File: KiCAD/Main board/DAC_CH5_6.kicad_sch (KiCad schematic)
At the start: 51 parts, among them U1 PCM1789-Q1, U3 OPA1632DR, U4 OPA1632DR

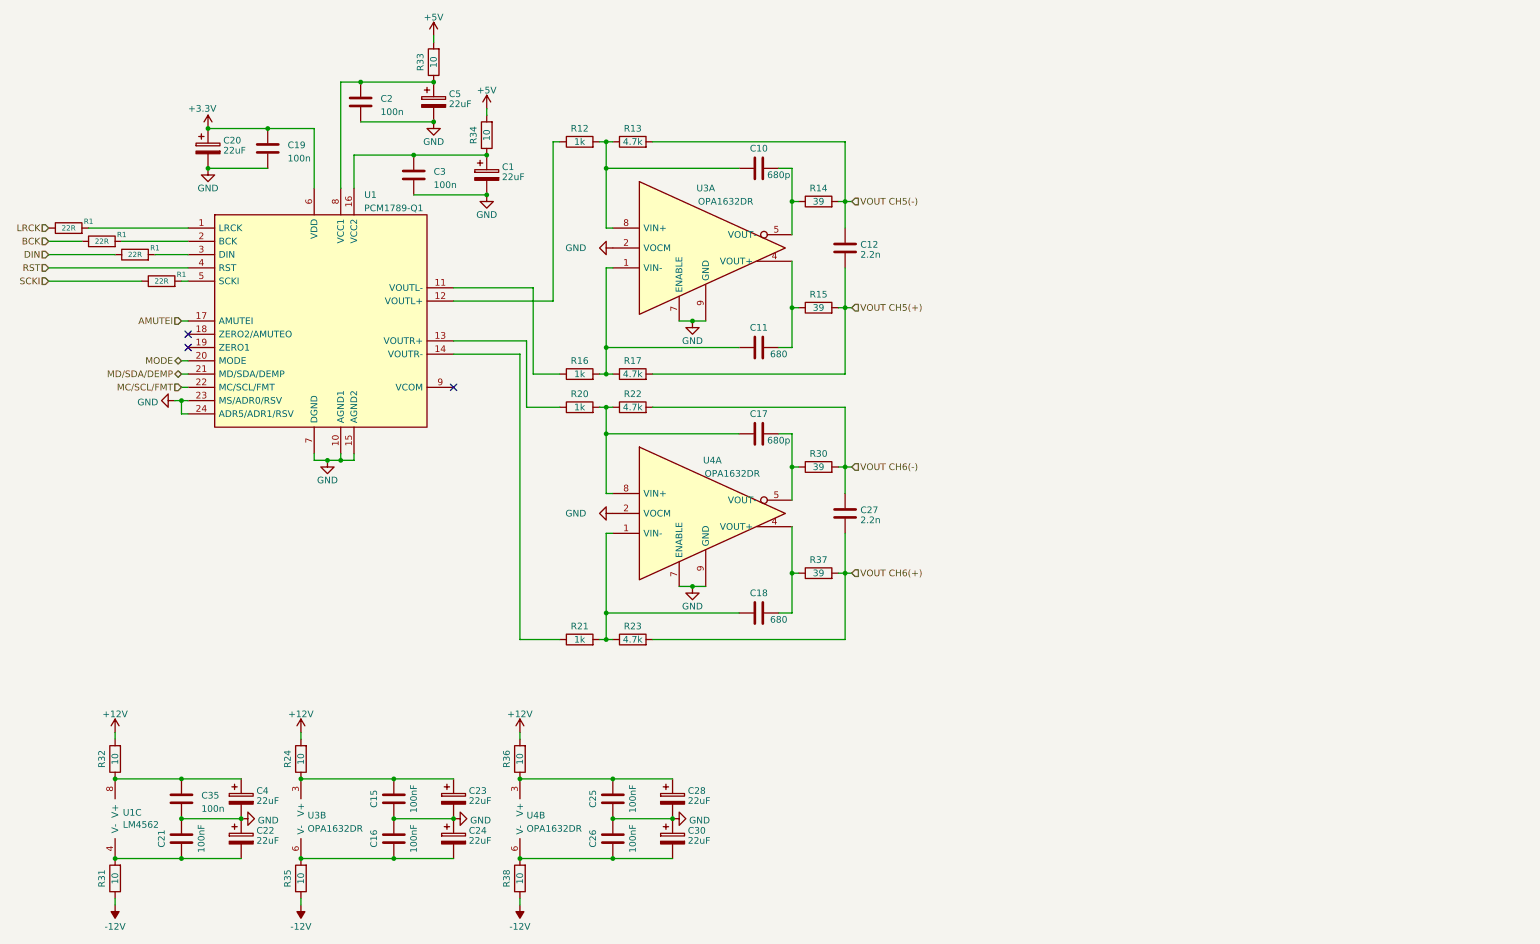
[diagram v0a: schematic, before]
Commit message: Worked a bit on the main board
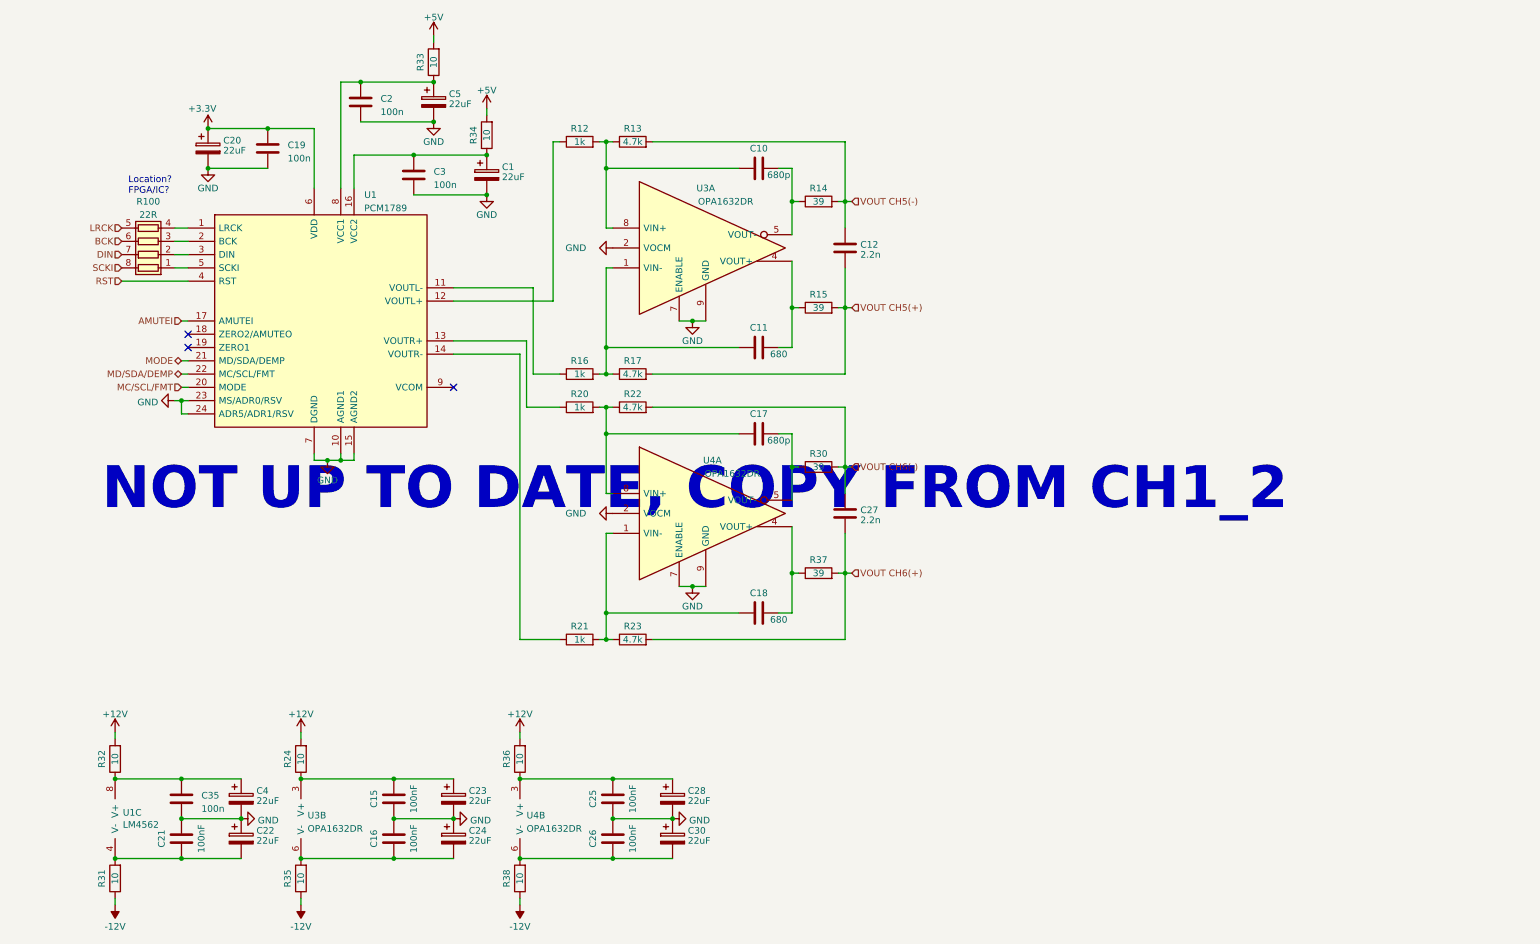
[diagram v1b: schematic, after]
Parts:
- removed R1 (x4): 22R, Resistor_SMD:R_0805_2012Metric, symbol Device:R
- removed unit 1 of U1
- added R100: 22R, Resistor_SMD:R_Array_Convex_4x0402, symbol Device:R_Pack04
- added unit 1 of U1
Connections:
- net +3.3V: now also U1.6 (VDD)
- net AMUTEI: now also U1.17 (AMUTEI)
- net BCK: now also R100.6 (R3.2)
- net DIN: now also R100.7 (R2.2)
- net GND: now also U1.10 (AGND1), U1.15 (AGND2), U1.23 (MS/ADR0/RSV), U1.24 (ADR5/ADR1/RSV), U1.7 (DGND)
- net LRCK: now also R100.5 (R4.2)
- net MC/SCL/FMT: now also U1.20 (MODE)
- net MD/SDA/DEMP: now also U1.22 (MC/SCL/FMT)
- net MODE: now also U1.21 (MD/SDA/DEMP)
- net RST: now also U1.4 (RST)
- net SCKI: now also R100.8 (R1.2)
- net at C1.1, C3.1, R34.1: now also U1.16 (VCC2)
- net at R20.1: now also U1.13 (VOUTR+)
- net at C2.1, C5.1, R33.1: now also U1.8 (VCC1)
- net at R21.1: now also U1.14 (VOUTR-)
- net at R16.1: now also U1.11 (VOUTL-)
- net at R12.1: now also U1.12 (VOUTL+)
- new net: R100.4 (R4.1), U1.1 (LRCK)
- new net: R100.3 (R3.1), U1.2 (BCK)
- new net: R100.2 (R2.1), U1.3 (DIN)
- new net: R100.1 (R1.1), U1.5 (SCKI)
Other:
- note added: "Location? FPGA/IC?"
- note added: "NOT UP TO DATE, COPY FROM CH1_2"

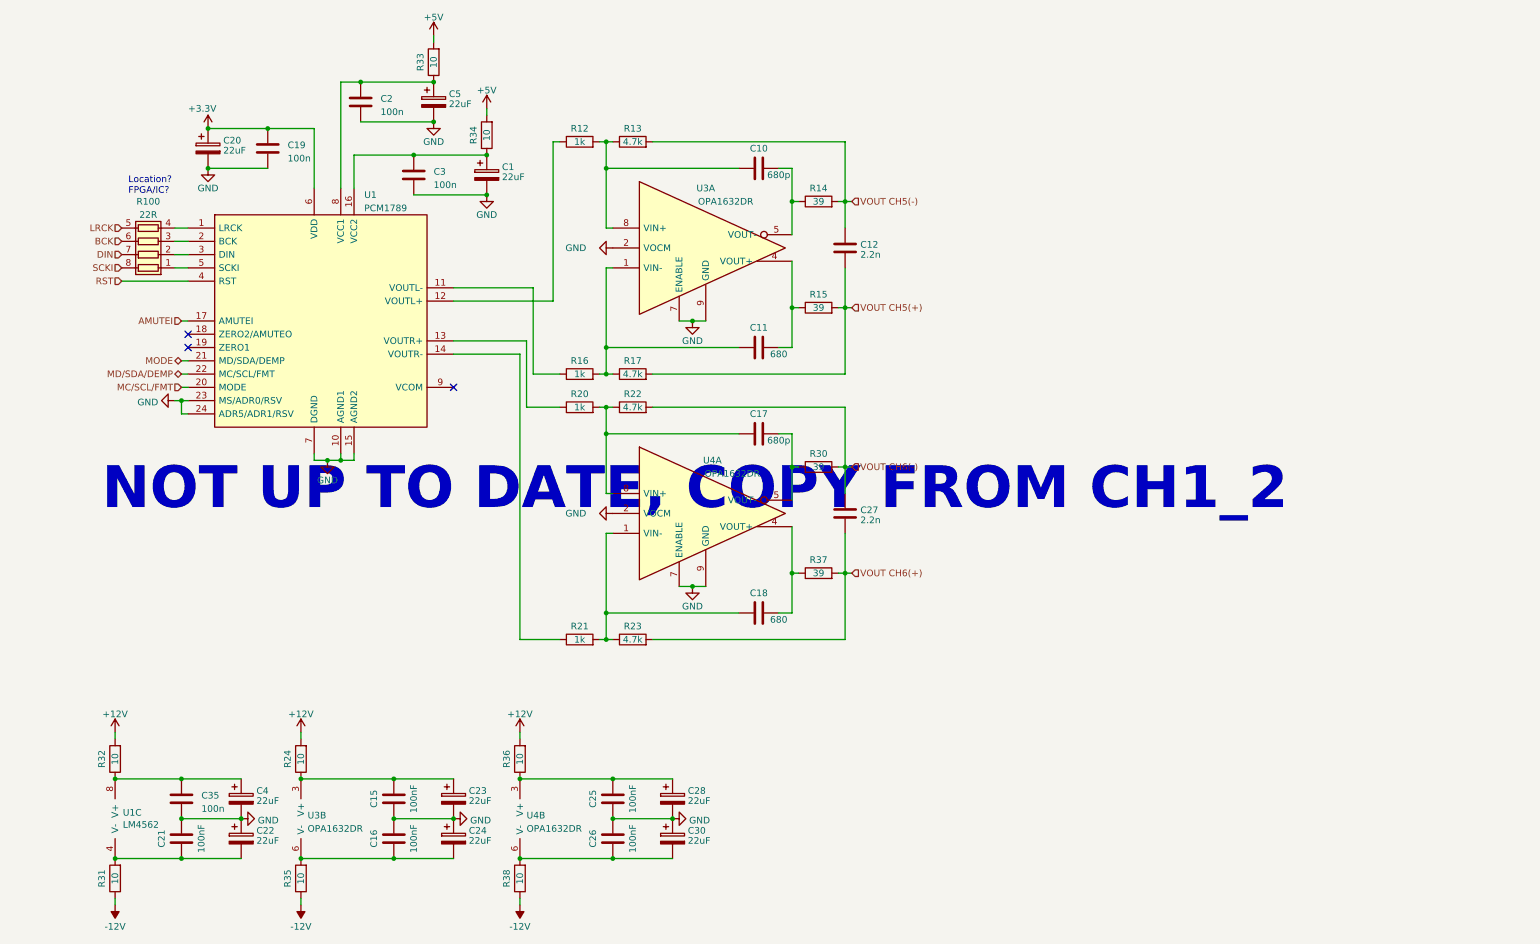
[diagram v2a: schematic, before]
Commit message: Worked on main board
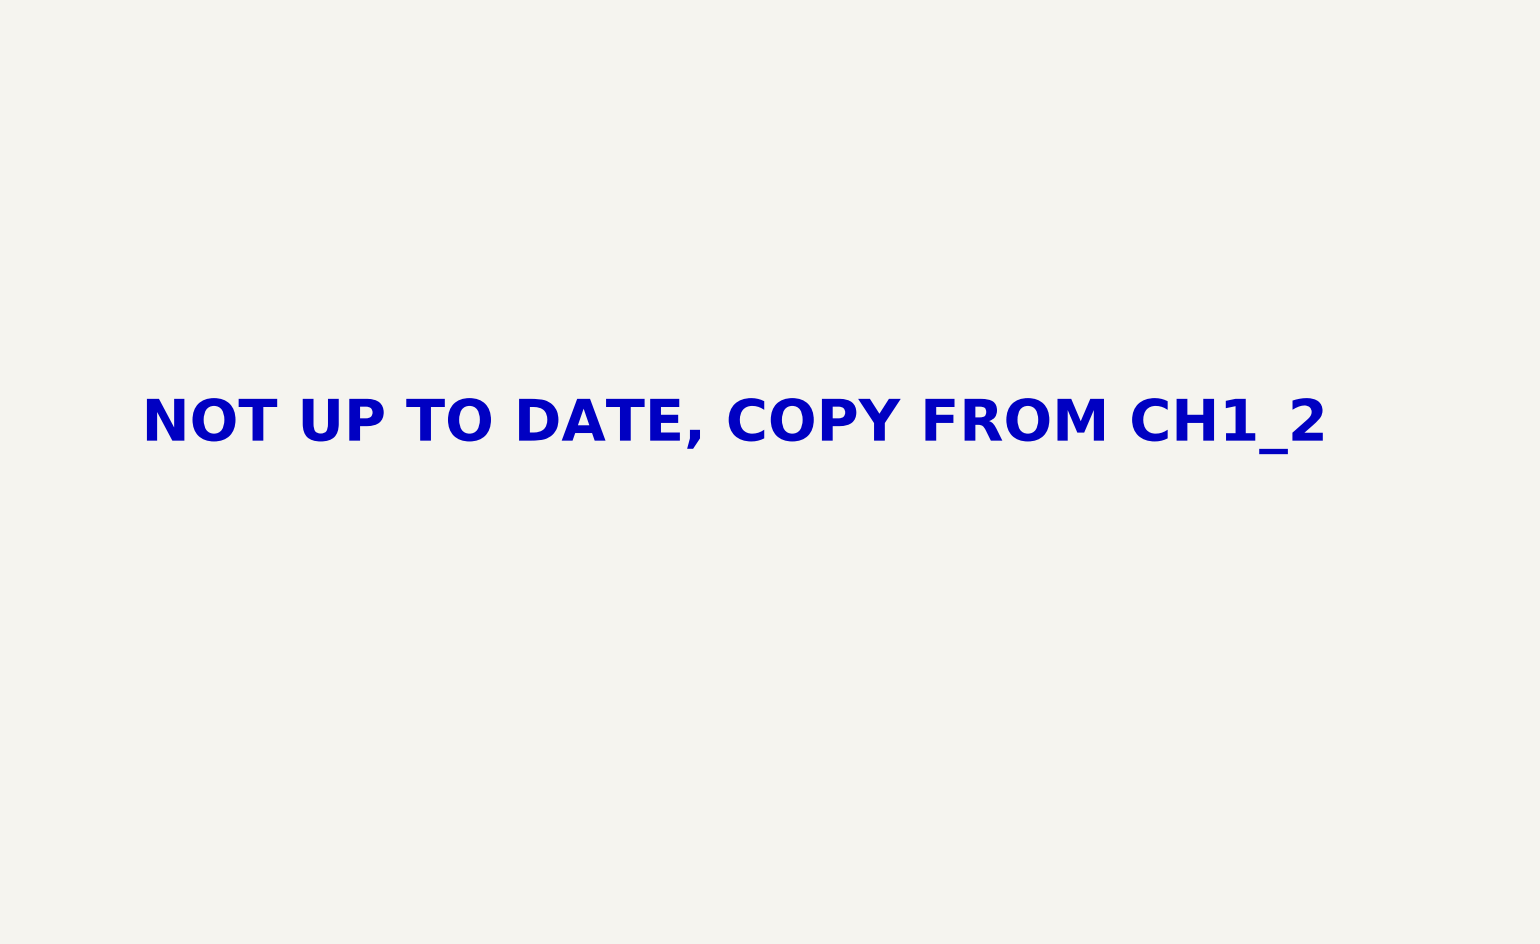
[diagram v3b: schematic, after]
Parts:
- removed C1, C20, C22, C23, C24, C28, C30, C4, C5: 22uF, Capacitor_THT:CP_Radial_D5.0mm_P2.00mm, symbol Device:C_Polarized
- removed C10, C17: 680p, Capacitor_SMD:C_0805_2012Metric, symbol Device:C
- removed C11, C18: 680, Capacitor_SMD:C_0805_2012Metric, symbol Device:C
- removed C12, C27: 2.2n, Capacitor_SMD:C_0805_2012Metric, symbol Device:C
- removed C15, C16, C21, C25, C26: 100nF, Capacitor_SMD:C_0805_2012Metric, symbol Device:C
- removed C19, C2, C3, C35: 100n, Capacitor_SMD:C_0805_2012Metric, symbol Device:C
- removed R100: 22R, Resistor_SMD:R_Array_Convex_4x0402, symbol Device:R_Pack04
- removed R12, R16, R20, R21: 1k, Resistor_SMD:R_0805_2012Metric, symbol Device:R
- removed R13, R17, R22, R23: 4.7k, Resistor_SMD:R_0805_2012Metric, symbol Device:R
- removed R14, R15, R30, R37: 39, Resistor_SMD:R_0805_2012Metric, symbol Device:R
- removed R24, R31, R32, R33, R34, R35, R36, R38: 10, Resistor_SMD:R_0805_2012Metric, symbol Device:R
- removed U1: PCM1789, Package_SO:TSSOP-24_4.4x7.8mm_P0.65mm, symbol Audio-DSP:PCM1789
- removed U3, U4: OPA1632DR, Audio_DSP:VSSOP-8_3.0x3.0mm_P0.65_TP1.8x1.5, symbol Audio-DSP:OPA1632DR
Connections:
- no-connect marks 3 -> 0
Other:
- note removed: "Location? FPGA/IC?"
